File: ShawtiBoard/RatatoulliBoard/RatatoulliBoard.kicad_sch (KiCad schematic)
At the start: 52 parts, among them IC1 TEENSY_4.1, IC2 DRV8212DRLR, IC3 DRV8212DRLR, J1 BDC1, J10 LINE_RB, J11 LINE_LB, J2 BDC2, J3 LIDAR1, J4 LIDAR2, J5 LIDAR3, J6 LIDAR4, J7 LINE_RF, J8 LINE_LF, J9 Battery, U1 ADP2303ARDZ-R7, U2 ADP2303ARDZ-R7

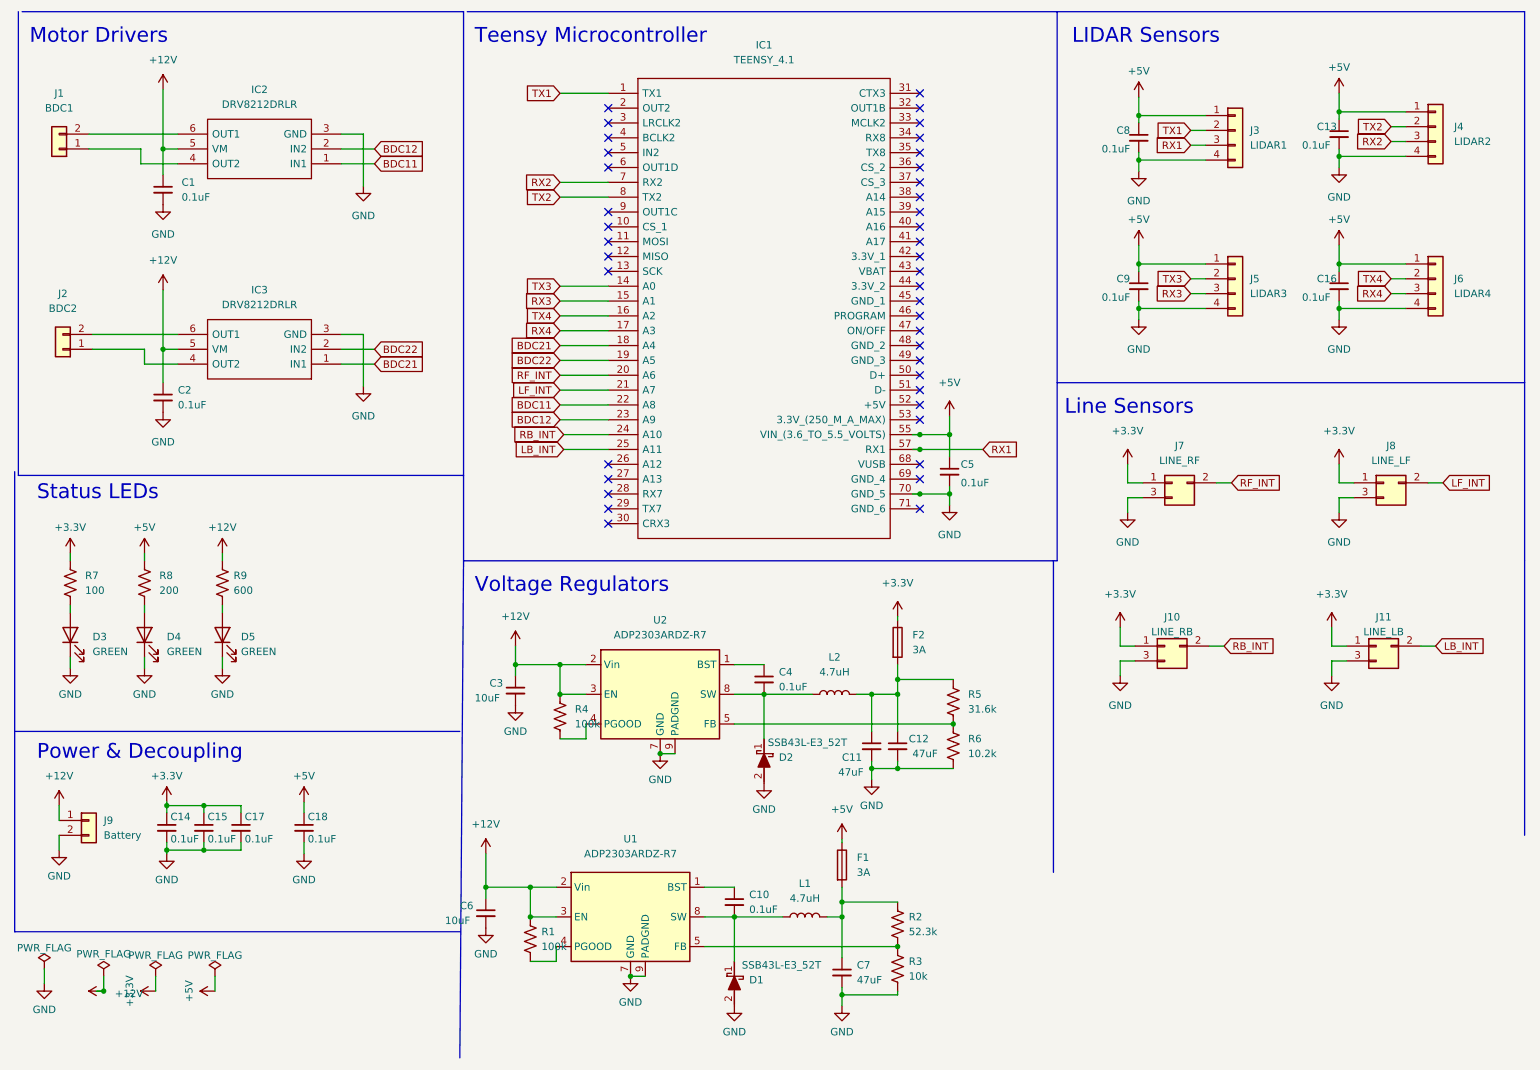
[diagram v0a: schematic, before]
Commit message: updates to 500g
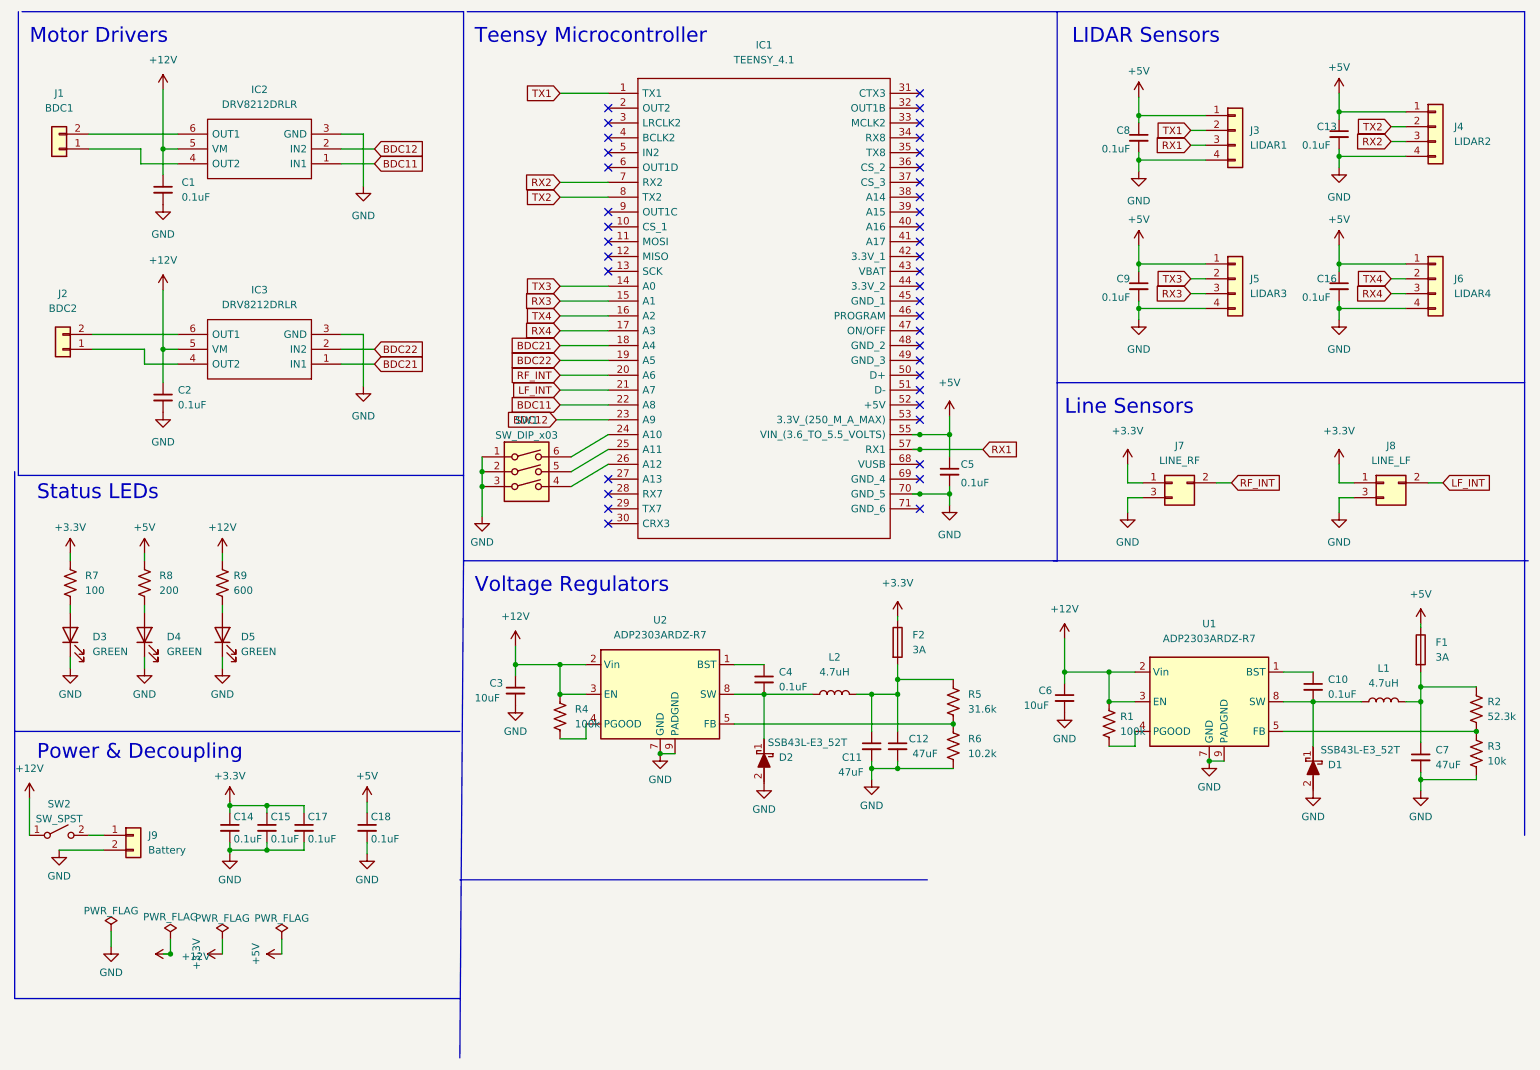
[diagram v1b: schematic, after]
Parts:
- removed J10: LINE_RB, phoenix:PhoenixContact_MSTBA_2,5_3-G_1x03_P5.00mm_Horizontal, symbol Connector_Generic:Conn_02x02_Odd_Even
- removed J11: LINE_LB, phoenix:PhoenixContact_MSTBA_2,5_3-G_1x03_P5.00mm_Horizontal, symbol Connector_Generic:Conn_02x02_Odd_Even
- added SW1: SW_DIP_x03, Button_Switch_SMD:SW_DIP_SPSTx03_Slide_9.78x9.8mm_W8.61mm_P2.54mm, symbol Switch:SW_DIP_x03
- added SW2: SW_SPST, Button_Switch_SMD:SW_SPST_B3S-1100, symbol Switch:SW_SPST
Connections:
- net +12V: now also SW2.1 (A); no longer J9.1 (Pin_1)
- net GND: now also SW1.1, SW1.2, SW1.3
- net at IC1.26 (A12): now also SW1.4
- net LB_INT: no longer names the net of IC1.25 (A11)
- net LB_INT: now also SW1.5
- net RB_INT: no longer names the net of IC1.24 (A10)
- net RB_INT: now also SW1.6
- new net: J9.1 (Pin_1), SW2.2 (B)
- no-connect marks 41 -> 40
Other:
- moved on the sheet: C10, C14, C15, C17, C18, C6, C7, D1, F1, J9, L1, R1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
